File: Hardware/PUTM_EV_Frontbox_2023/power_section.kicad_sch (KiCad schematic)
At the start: 20 parts, among them U4 MIC94310-SYM5-TR, U5 MIC94310-SYM5-TR, U6 BD50FC0FP, U7 MIC94310-SYM5-TR

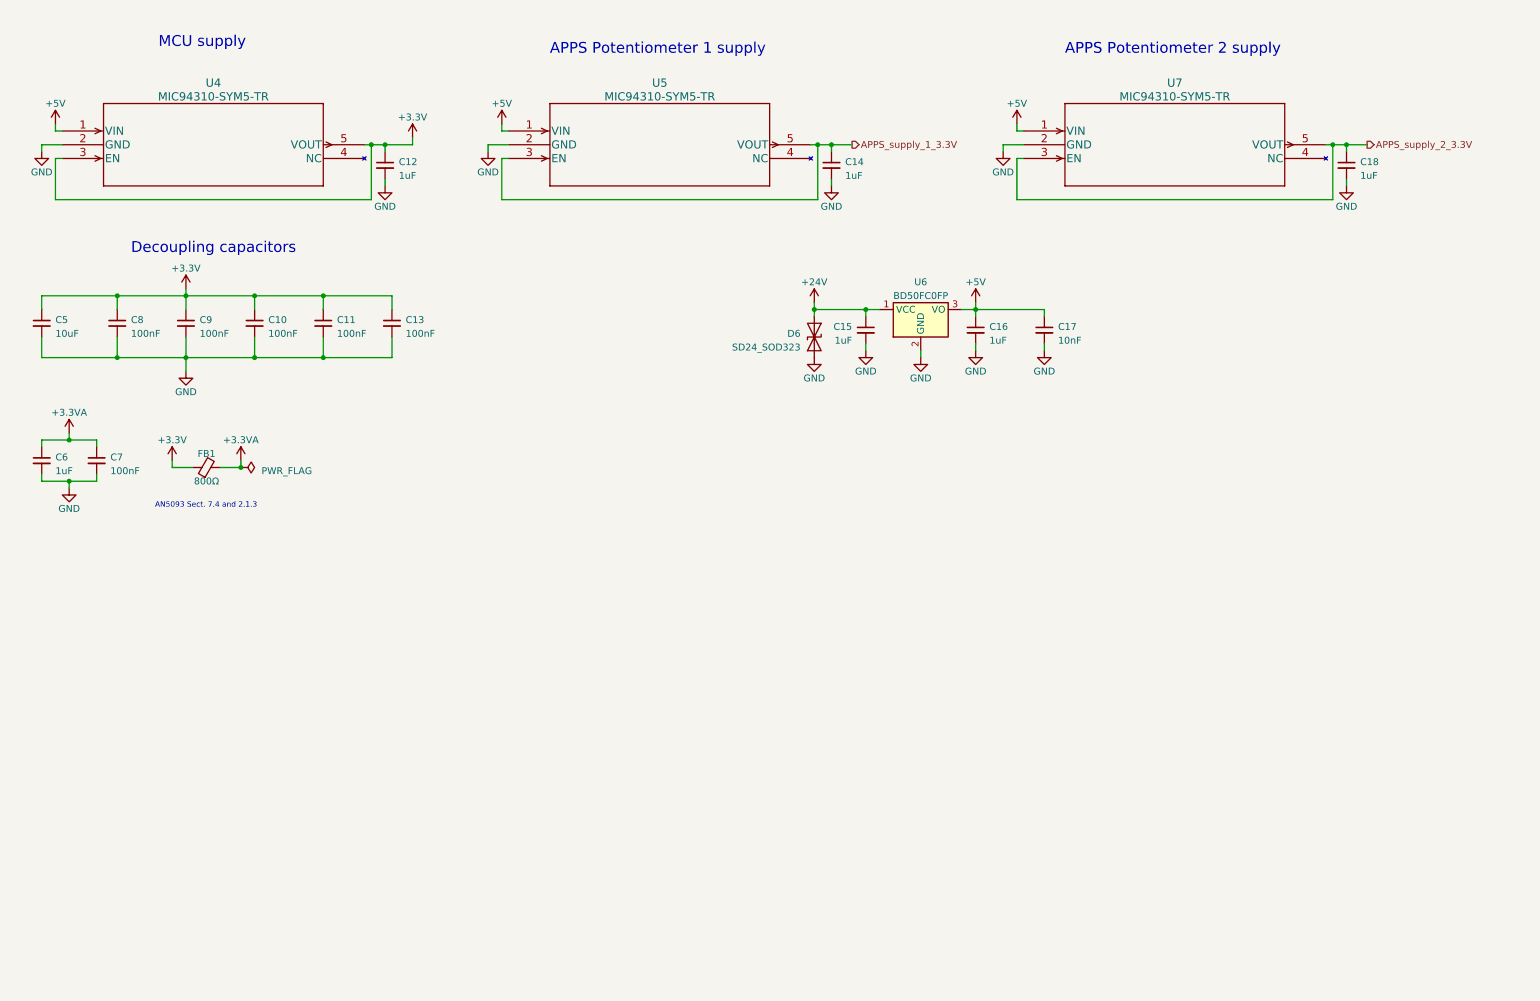
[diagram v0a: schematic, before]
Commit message: Fixed all issues
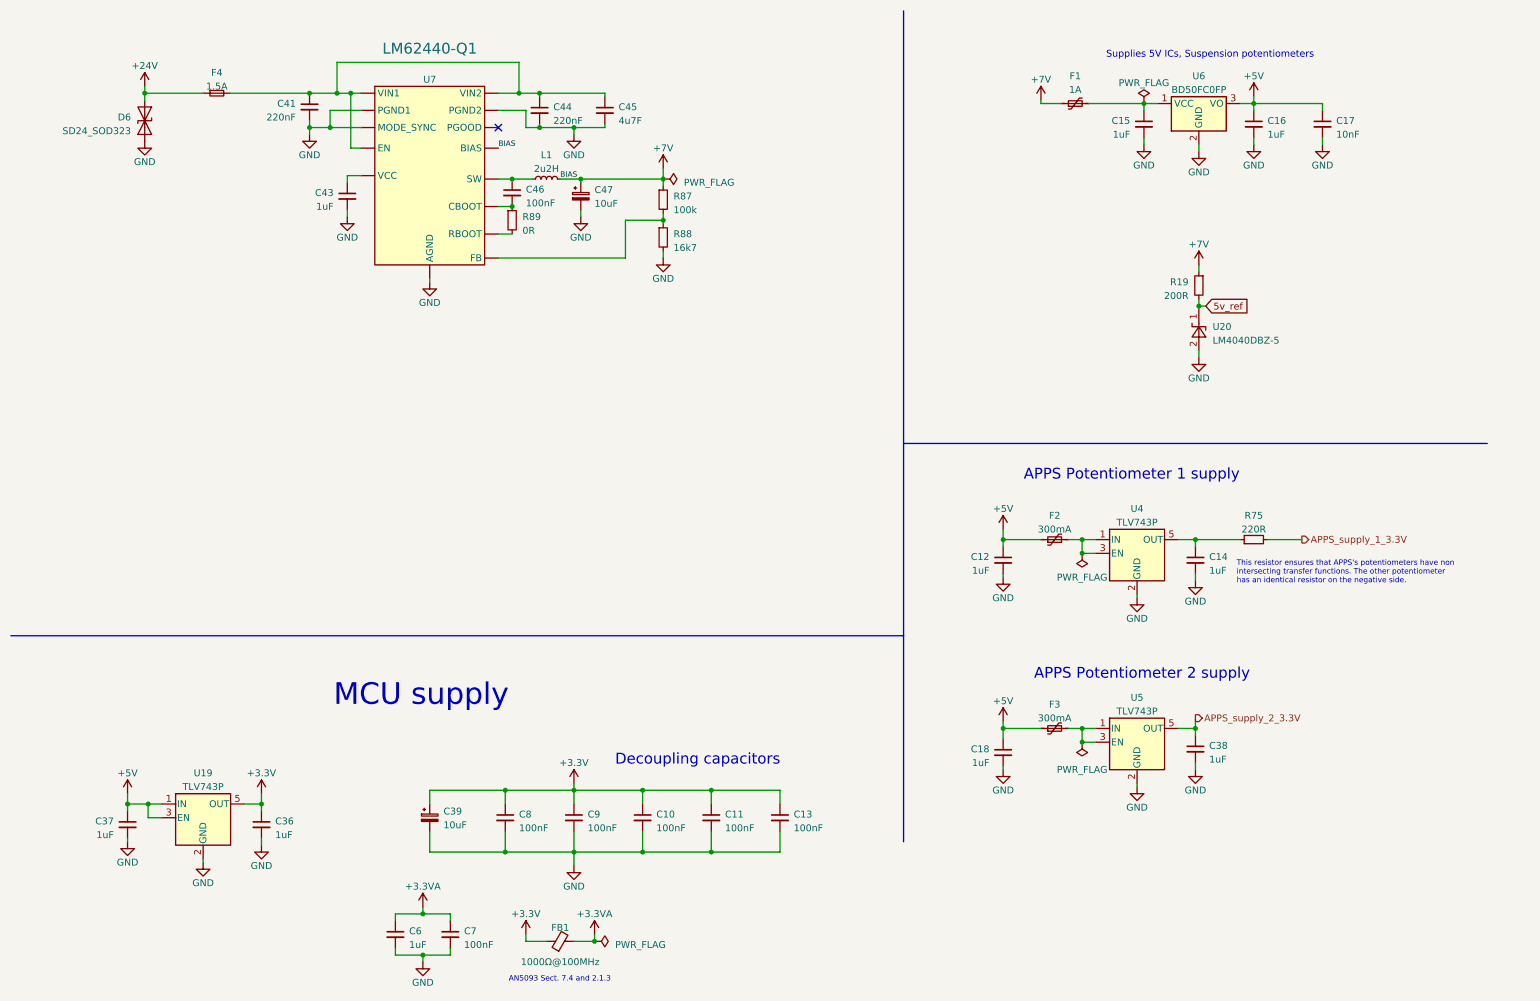
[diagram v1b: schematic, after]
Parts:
- removed C5: 10uF, symbol Device:C_Small
- removed U4, U5, U7: MIC94310-SYM5-TR, SOT-23-5_M5_MCH, symbol ul_MIC94310-SYM5-TR:MIC94310-SYM5-TR
- added C36, C37, C38, C43: 1uF, symbol Device:C_Small
- added C39, C47: 10uF, symbol Device:C_Polarized_Small
- added C41, C44: 220nF, symbol Device:C_Small
- added C45: 4u7F, symbol Device:C_Small
- added C46: 100nF, symbol Device:C_Small
- added F1: 1A, symbol Device:Polyfuse_Small
- added F2, F3: 300mA, symbol Device:Polyfuse_Small
- added F4: 1.5A, symbol Device:Fuse_Small
- added L1: 2u2H, symbol Device:L_Small
- added R19: 200R, symbol Device:R_Small
- added R75: 220R, symbol Device:R_Small
- added R87: 100k, symbol Device:R_Small
- added R88: 16k7, symbol Device:R_Small
- added R89: 0R, symbol Device:R_Small
- added U19, U4, U5: TLV743P, symbol Regulator_Linear:TLV73330PDBV
- added U20: LM4040DBZ-5, Package_TO_SOT_SMD:SOT-23, symbol Reference_Voltage:LM4040DBZ-5
- added U7: LM62440-Q1, symbol LMR51420:LM62440
- FB1: value 800Ω -> 1000Ω@100MHz
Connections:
- net +24V: now also F4.1; no longer C15.1, U6.1 (VCC)
- net +3.3V: now also C36.1, C39.1, U19.5 (OUT); no longer C12.1
- net +5V: now also C12.1, C18.1, C37.1, F2.1, F3.1, U19.1 (IN), U19.3 (EN)
- net APPS_supply_1_3.3V: now also R75.2; no longer C14.1
- net APPS_supply_2_3.3V: now also C38.1, U5.5 (OUT); no longer C18.1
- net GND: now also C36.2, C37.2, C38.2, C39.2, C41.2, C43.2, C44.2, C45.2, C47.2, R88.2, U19.2 (GND), U20.2 (A), U4.2 (GND), U5.2 (GND), U7. (VIN2)
- new net: C15.1, F1.2, U6.1 (VCC)
- new net: C41.1, C44.1, C45.1, F4.2, U7. (VIN2)
- new net: F3.2, U5.1 (IN), U5.3 (EN)
- new net: C14.1, R75.1, U4.5 (OUT)
- new net: C46.1, L1.1, U7. (VIN2)
- new net: F2.2, U4.1 (IN), U4.3 (EN)
- new net: C46.2, R89.1, U7. (VIN2)
- new net: C43.1, U7. (VIN2)
- new net: R87.2, R88.1, U7. (VIN2)
- new net: R89.2, U7. (VIN2)
- new net +7.5V: C47.1, F1.1, L1.2, R19.1, R87.1, U7. (VIN2)
- new net 5v_ref: R19.2, U20.1 (K)
- no-connect marks 0 -> 1
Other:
- note added: "Supplies 5V ICs, Suspension potentiometers"
- note added: "This resistor ensures that APPS's potentiometers have non intersecting transfer functions. The other potentiometer has an identical resistor on the negative side."
- moved on the sheet: C10, C11, C13, C15, C16, C17, C6, C7, C8, C9, D6, FB1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
